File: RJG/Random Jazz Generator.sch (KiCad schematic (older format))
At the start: 19 parts, among them J101 EuroPower, J102 CV, J103 RND, J104 Gate, J105 Trig1, J106 Trig2, J107 Clock, J108 Trig3, J109 Trig4, U101 4520, U102 L7805

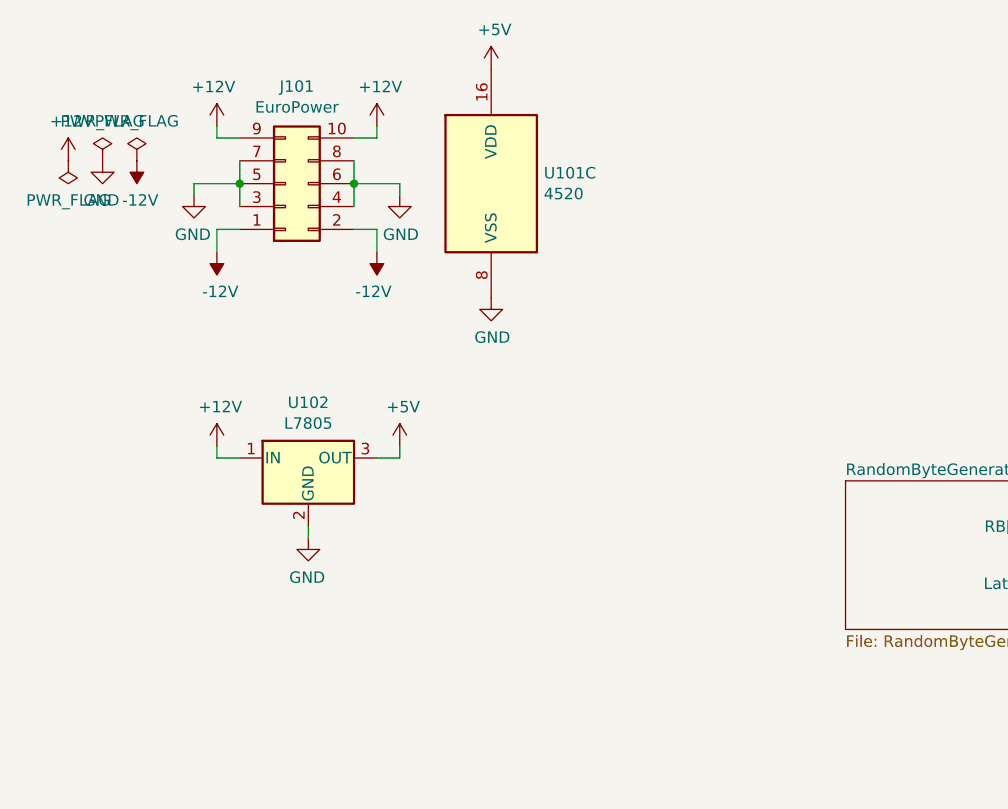
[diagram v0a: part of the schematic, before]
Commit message: Small improvements
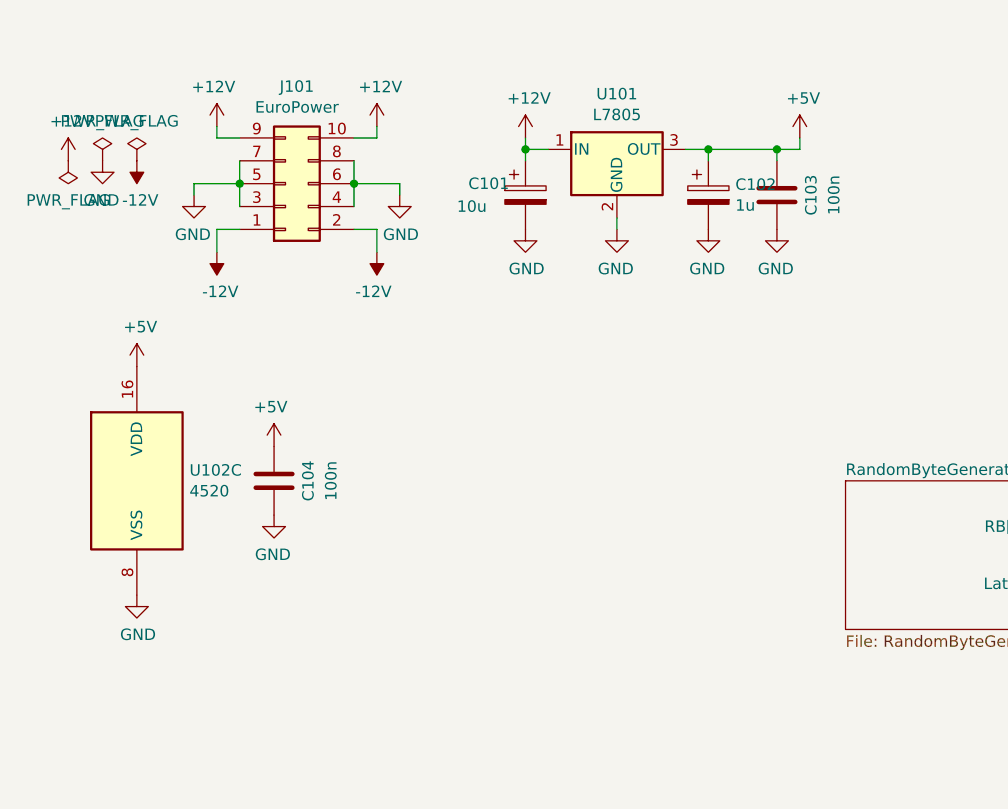
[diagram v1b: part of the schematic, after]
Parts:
- added C101: 10u, symbol Device:CP
- added C102: 1u, symbol Device:CP
- added C103, C104: 100n, Capacitor_THT:C_Disc_D7.0mm_W2.5mm_P5.00mm, symbol Device:C
- renumbered U102 to U101, U101 to U102
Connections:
- net +12V: now also C101.1
- net +5V: now also C102.1, C103.2, C104.2
- net GND: now also C101.2, C102.2, C103.1, C104.1
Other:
- moved on the sheet: U101, U102C
